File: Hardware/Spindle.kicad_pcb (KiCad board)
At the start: 4 copper layers, 50 x 40 mm, 54 parts, among them J1 USB_C_Receptacle_USB2.0_16P, J2 Conn_01x02_Pin, J3 Conn_01x24_Pin, J4 Micro_SD_Card, Q1 Si1308EDL, SW1 SW_Push, U1 RP2350A, U2 BQ24074RGT, U3 MCP1700x-330xxTT, U4 W25Q128JVP, Y1 12mhz

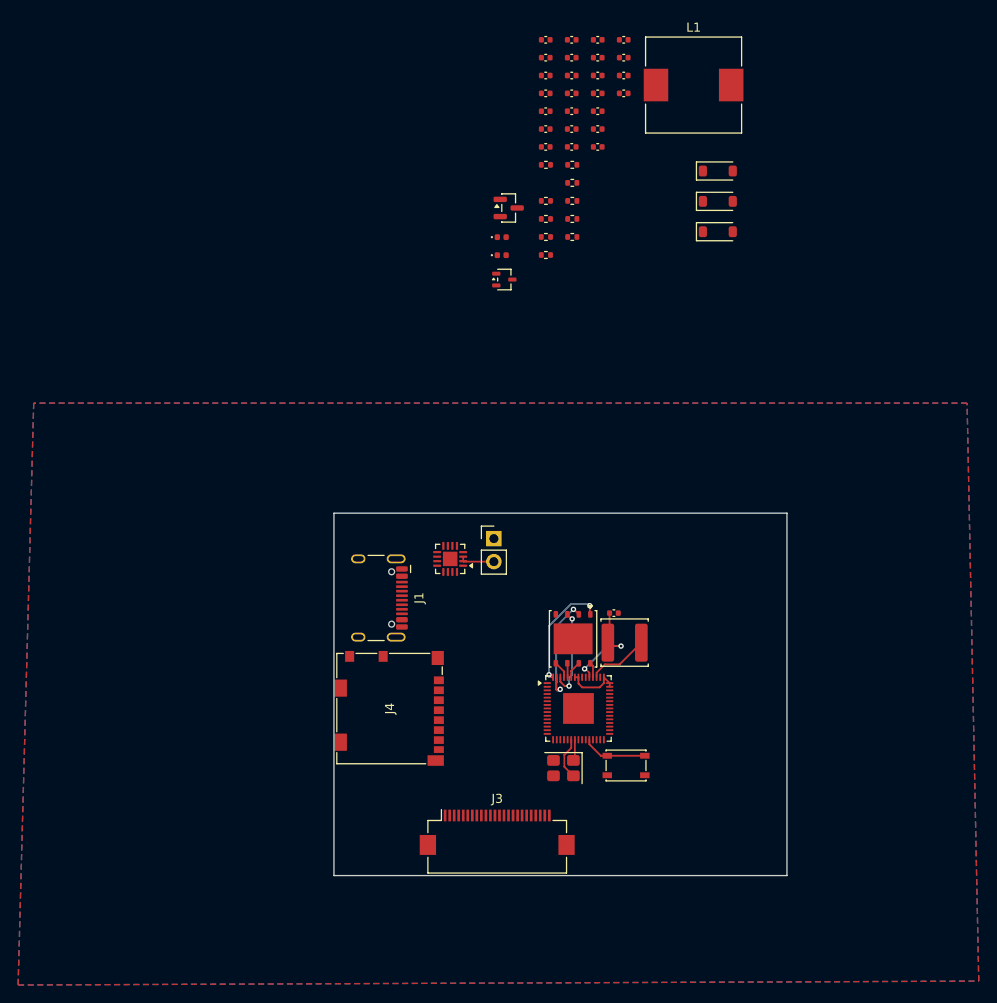
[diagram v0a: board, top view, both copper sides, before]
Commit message: Completed PCB
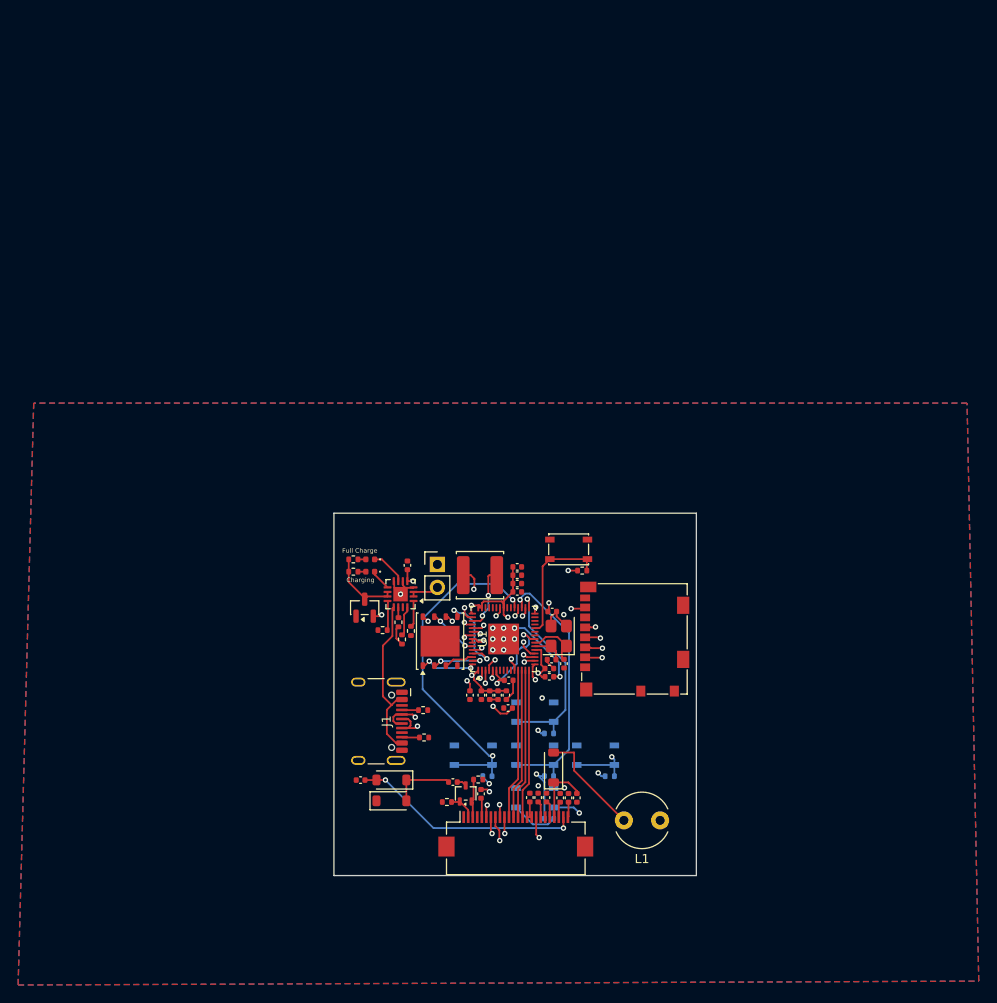
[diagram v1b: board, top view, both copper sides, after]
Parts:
- added R12: 10K, Resistor_SMD:R_0402_1005Metric, B.Cu at (447.6, 172.6)
- added R13: 10K, Resistor_SMD:R_0402_1005Metric, B.Cu at (440.8, 177.3)
- added R14: 10K, Resistor_SMD:R_0402_1005Metric, B.Cu at (447.6, 177.3)
- added R15: 10K, Resistor_SMD:R_0402_1005Metric, B.Cu at (447.6, 182.0)
- added R16: 10K, Resistor_SMD:R_0402_1005Metric, B.Cu at (454.3, 177.3)
- added R2: 10K, Resistor_SMD:R_0402_1005Metric, F.Cu at (432.3, 161.3)
- added SW2: SW_Push, Button_Switch_SMD:SW_SPST_PTS810, B.Cu at (446.0, 170.2)
- added SW3: SW_Push, Button_Switch_SMD:SW_SPST_PTS810, B.Cu at (439.2, 175.0)
- added SW4: SW_Push, Button_Switch_SMD:SW_SPST_PTS810, B.Cu at (446.0, 175.0)
- added SW5: SW_Push, Button_Switch_SMD:SW_SPST_PTS810, B.Cu at (446.0, 179.7)
- added SW6: SW_Push, Button_Switch_SMD:SW_SPST_PTS810, B.Cu at (452.7, 175.0)
- L1: footprint Inductor_SMD:L_10.4x10.4_H4.8 -> Inductor_THT:L_Radial_D6.0mm_P4.00mm
- moved C8 83.7 mm to (446.4, 179.7), turned to 90 degrees
- moved C9 81.7 mm to (447.3, 179.7), turned to 90 degrees
- moved L1 81.2 mm to (459.8, 182.2), turned to 180 degrees
- moved C10 79.7 mm to (448.8, 179.7), turned to 90 degrees
- moved C11 79.3 mm to (426.8, 177.7), turned to 180 degrees
- moved C3 78.7 mm to (436.9, 177.9)
- moved C4 77.8 mm to (450.6, 179.7), turned to -90 degrees
- moved D3 76.3 mm to (430.2, 177.7), turned to 180 degrees
- moved C12 75.8 mm to (449.7, 179.7), turned to 90 degrees
- moved D4 75.3 mm to (430.2, 180.0)
- moved C23 74.9 mm to (443.0, 169.8), turned to 180 degrees
- moved C6 73.7 mm to (440.1, 179.2), turned to 90 degrees
- moved C15 73.2 mm to (441.9, 168.4), turned to -90 degrees
- moved C7 71.8 mm to (445.4, 179.7), turned to 90 degrees
- moved C16 71.4 mm to (441.0, 168.4), turned to -90 degrees
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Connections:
- J3 pad : GND -> (no net)
- J4 pad : GND -> (no net)
- U1 pad 31: unconnected-(U1-GPIO19-Pad31) -> /SW_UP
- U1 pad 32: unconnected-(U1-GPIO20-Pad32) -> /SW_DOWN
- U1 pad 33: unconnected-(U1-GPIO21-Pad33) -> /SW_CENTRE
- U1 pad 34: unconnected-(U1-GPIO22-Pad34) -> /SW_RIGHT
- U1 pad 35: unconnected-(U1-GPIO23-Pad35) -> /SW_LEFT
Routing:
- net +3V3: track 7.90 -> 59.6 mm, vias 0 -> 19
- net /SW_DOWN: track 0.00 -> 38.5 mm, vias 0 -> 2
- net /SW_LEFT: track 0.00 -> 38.2 mm, vias 0 -> 2
- net GND: track 0.00 -> 30.1 mm, vias 0 -> 17
- net /SW_CENTRE: track 0.00 -> 29.2 mm, vias 0 -> 1
- net /SW_RIGHT: track 0.00 -> 27.7 mm, vias 0 -> 2
- net /DATA-: track 0.00 -> 26.1 mm, vias 0 -> 2
- net /VGL: track 0.00 -> 25.3 mm, vias 0 -> 2
- net /TP_SDA: track 0.00 -> 24.4 mm, vias 0 -> 2
- net /SD_CLK: track 0.00 -> 23.6 mm, vias 0 -> 2
- net /TP_SCL: track 0.00 -> 23.3 mm, vias 0 -> 2
- net /DVDD: track 0.00 -> 22.7 mm, vias 0 -> 4
- net /DATA+: track 0.00 -> 22.4 mm, vias 0 -> 2
- net /SW_UP: track 0.00 -> 22.3 mm, vias 0 -> 1
- net /EPD_RST: track 0.00 -> 22.1 mm, vias 0 -> 2
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- added copper zone on In1.Cu, net +3V3
- added copper zone on In2.Cu, net GND
- removed copper zone on In1.Cu, net GND
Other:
- board size 50 x 40 mm -> 40 x 40 mm
- board text added: "Charging"
- board text added: "Full Charge"
